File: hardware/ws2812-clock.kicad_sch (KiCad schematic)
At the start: 36 parts, among them J1 Conn_01x01_Pin, Q3 2N7002, Q5 AO4485, SW2 Reset ESP, SW5 Toggle AP, SW6 Toggle Alarm, SW7 Snooze Alarm, U1 ESP32-WROOM-32D, U3 SHT30-DIS, U4 AMS1117-3.3, U5 BME280

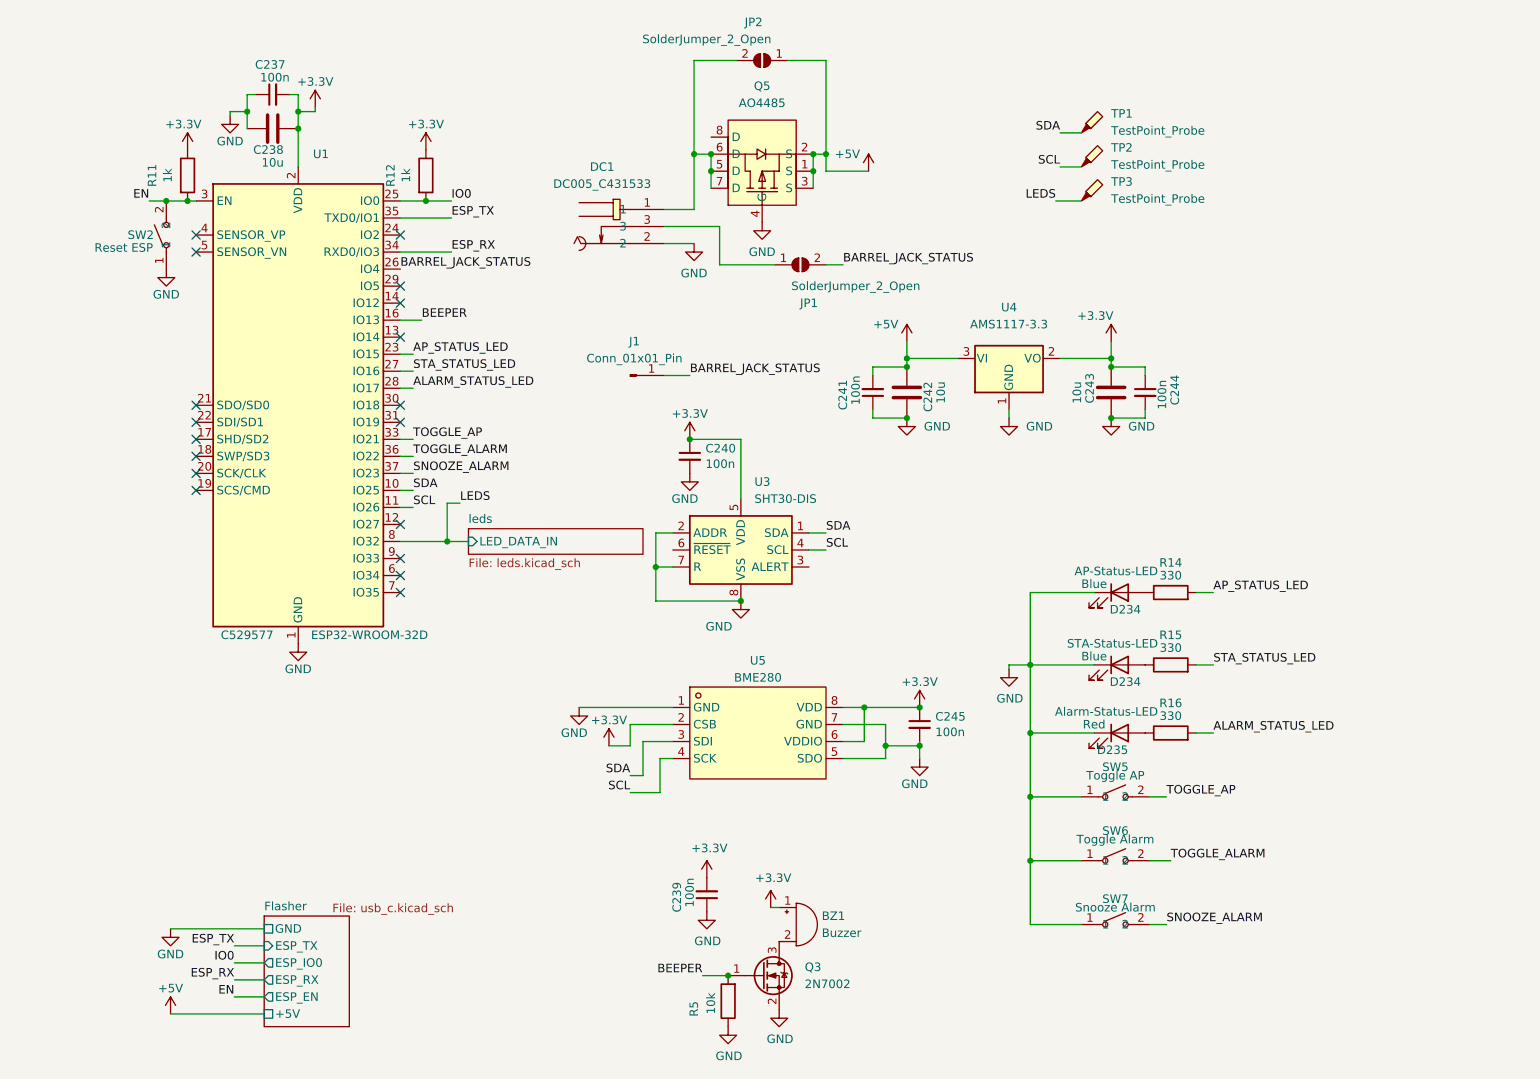
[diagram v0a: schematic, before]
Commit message: PCB rework (ordered)
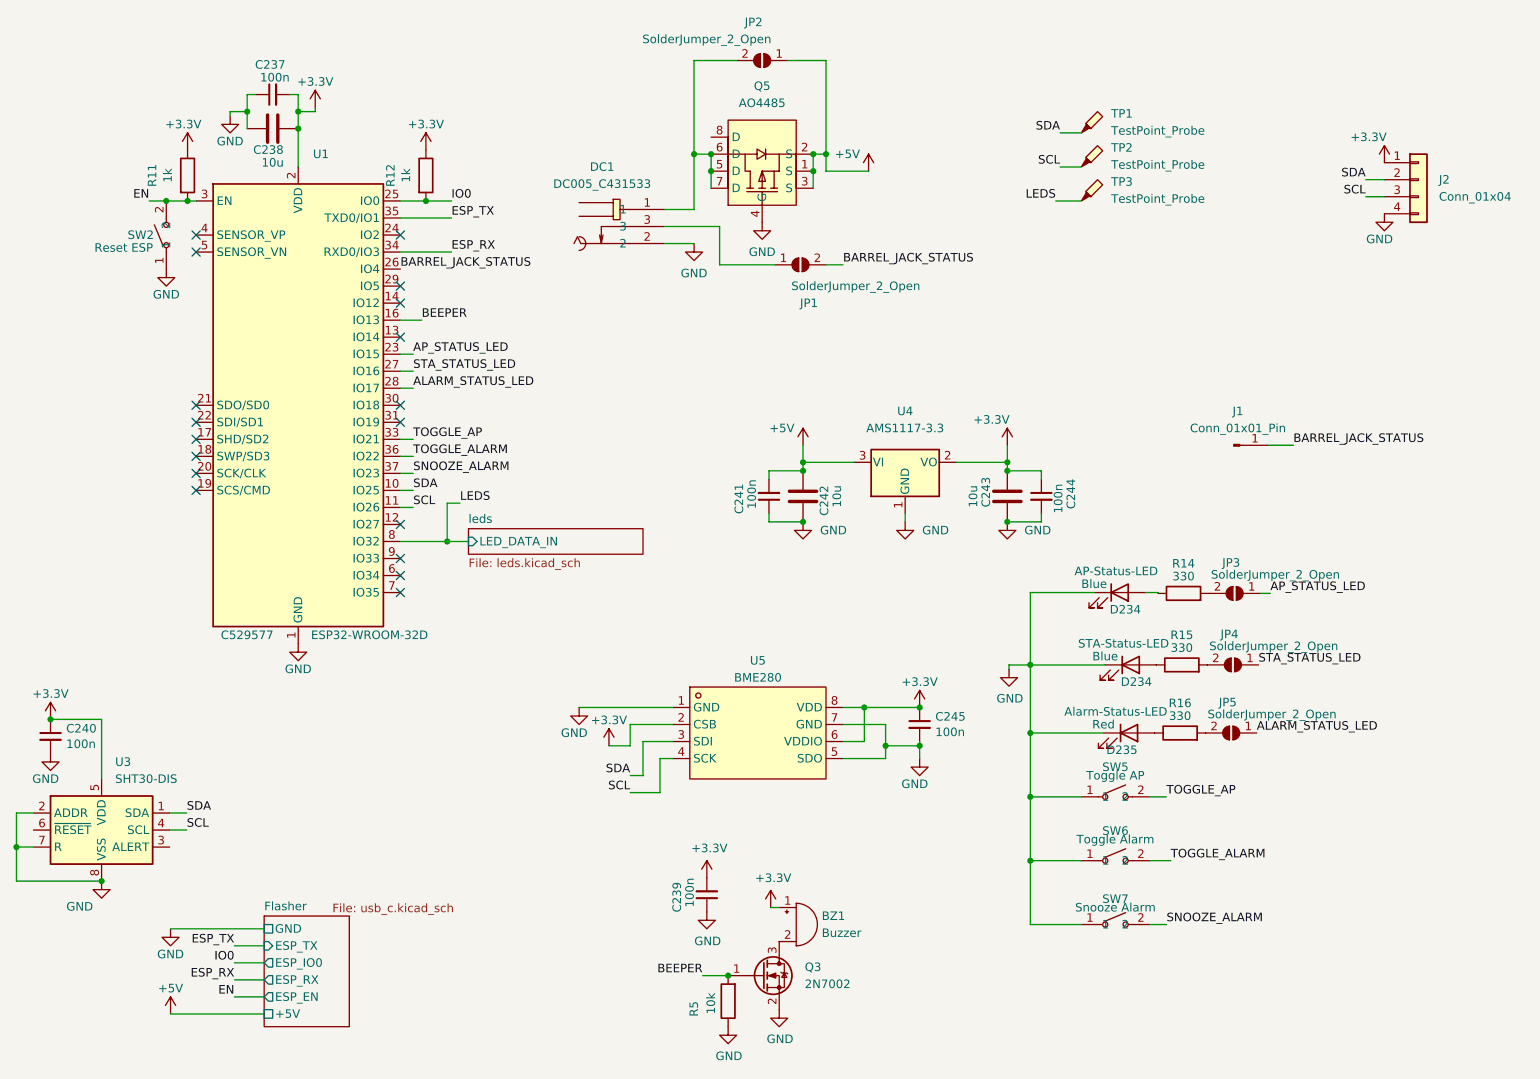
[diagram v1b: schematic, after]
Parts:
- added J2: Conn_01x04, Connector_PinHeader_2.54mm:PinHeader_1x04_P2.54mm_Vertical, symbol Connector_Generic:Conn_01x04
- added JP3, JP4, JP5: SolderJumper_2_Open, Jumper:SolderJumper-2_P1.3mm_Open_TrianglePad1.0x1.5mm, symbol Jumper:SolderJumper_2_Open
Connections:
- net +3.3V: now also J2.1 (Pin_1)
- net ALARM_STATUS_LED: now also JP5.1 (A); no longer R16.2
- net AP_STATUS_LED: now also JP3.1 (A); no longer R14.2
- net GND: now also J2.4 (Pin_4)
- net SCL: now also J2.3 (Pin_3)
- net SDA: now also J2.2 (Pin_2)
- net STA_STATUS_LED: now also JP4.1 (A); no longer R15.2
- new net: JP3.2 (B), R14.2
- new net: JP5.2 (B), R16.2
- new net: JP4.2 (B), R15.2
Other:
- moved on the sheet: C240, C241, C242, C243, C244, D234, D235, J1, R14, R15, R16, U3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
